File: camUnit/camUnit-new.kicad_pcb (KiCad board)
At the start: 2 copper layers, 130 x 130 mm, 38 parts, among them J1 Conn_01x06, J2 Conn_01x06, J3 Conn_01x06, J4 Conn_01x06, J5 Conn_01x06, SW1 SW_SPDT, SW2 SW_SPDT, SW3 SW_SPDT, SW4 SW_SPDT, U2 BNO085, U3 xiao-esp32c3, U4 Teensy 4.0, U5 xiao-esp32c3

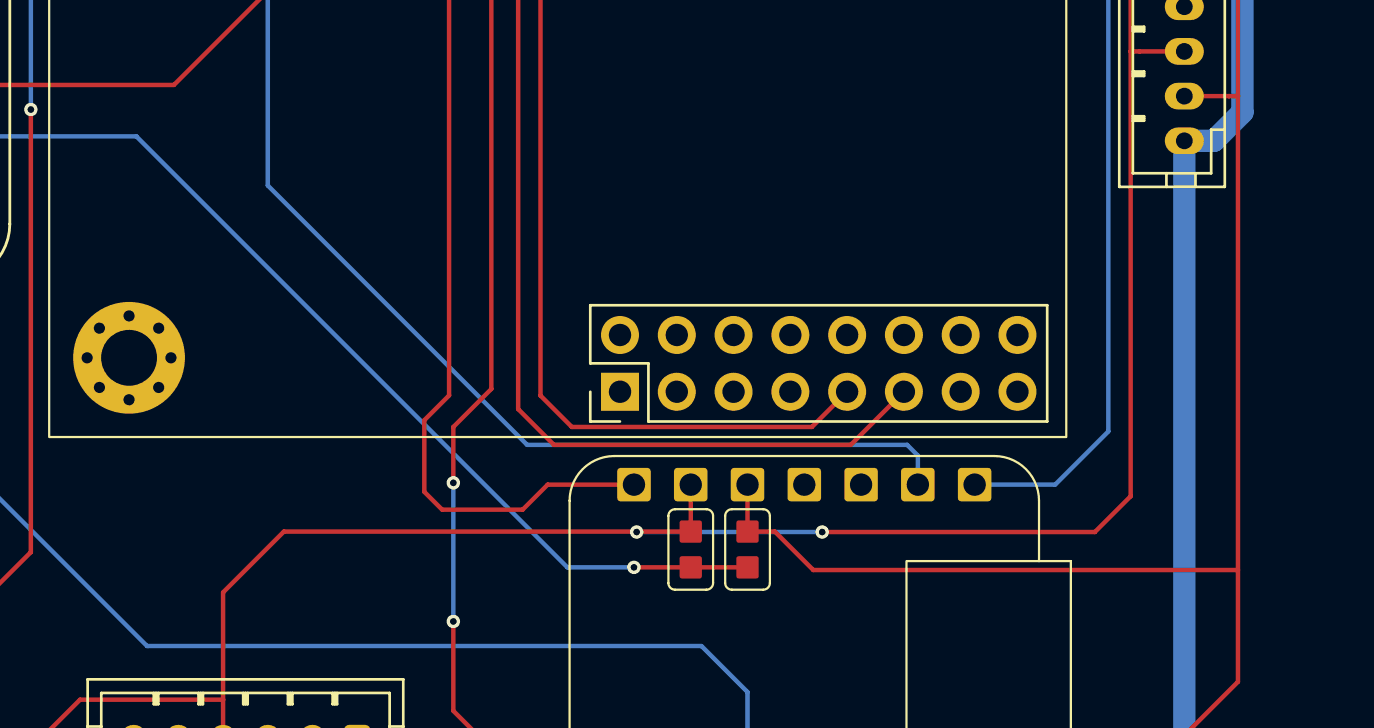
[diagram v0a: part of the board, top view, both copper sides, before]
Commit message: cam prod ready
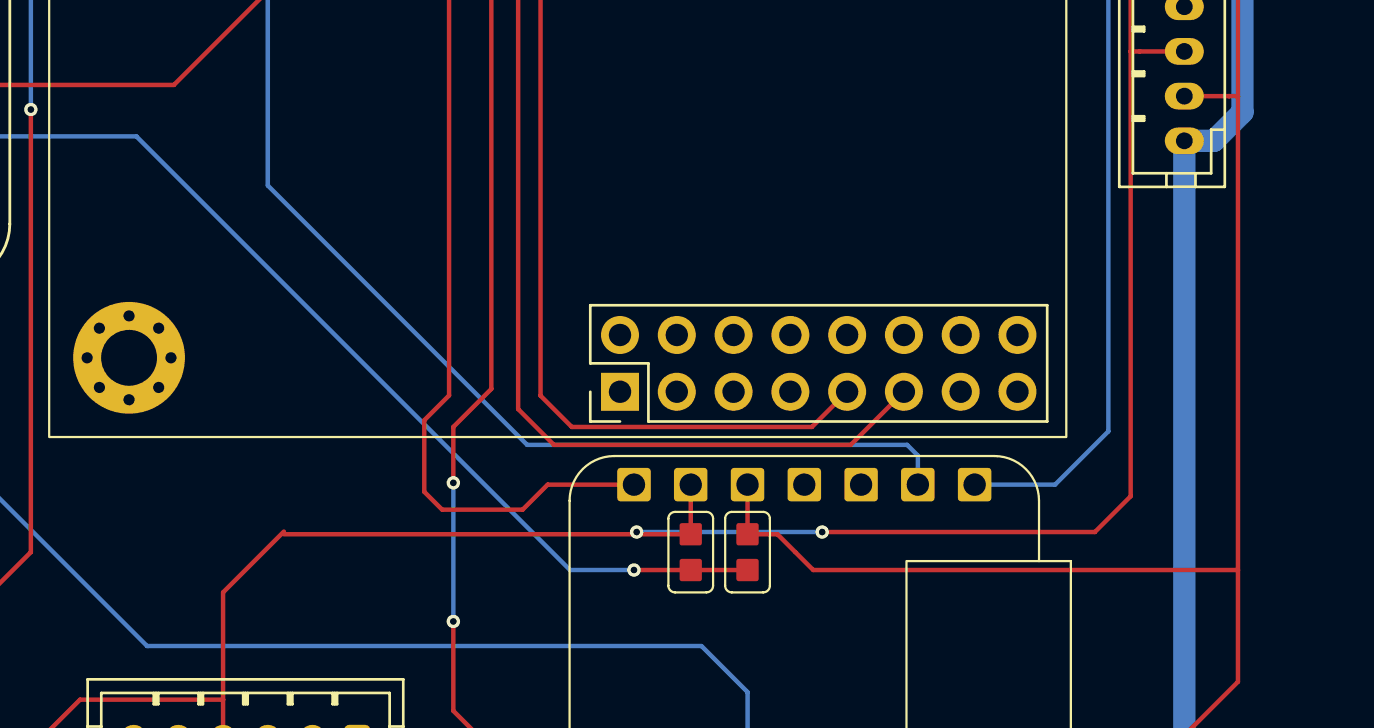
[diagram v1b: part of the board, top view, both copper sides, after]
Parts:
- U3, U5: value xiao-esp32c3 -> >VALUE
- moved R4 0.12 mm to (179.9, 123.4)
- moved R5 0.12 mm to (182.5, 123.4)
